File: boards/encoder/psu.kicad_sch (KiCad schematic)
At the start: 10 parts, among them J1 Conn_PWR, U2 TPS62A02A

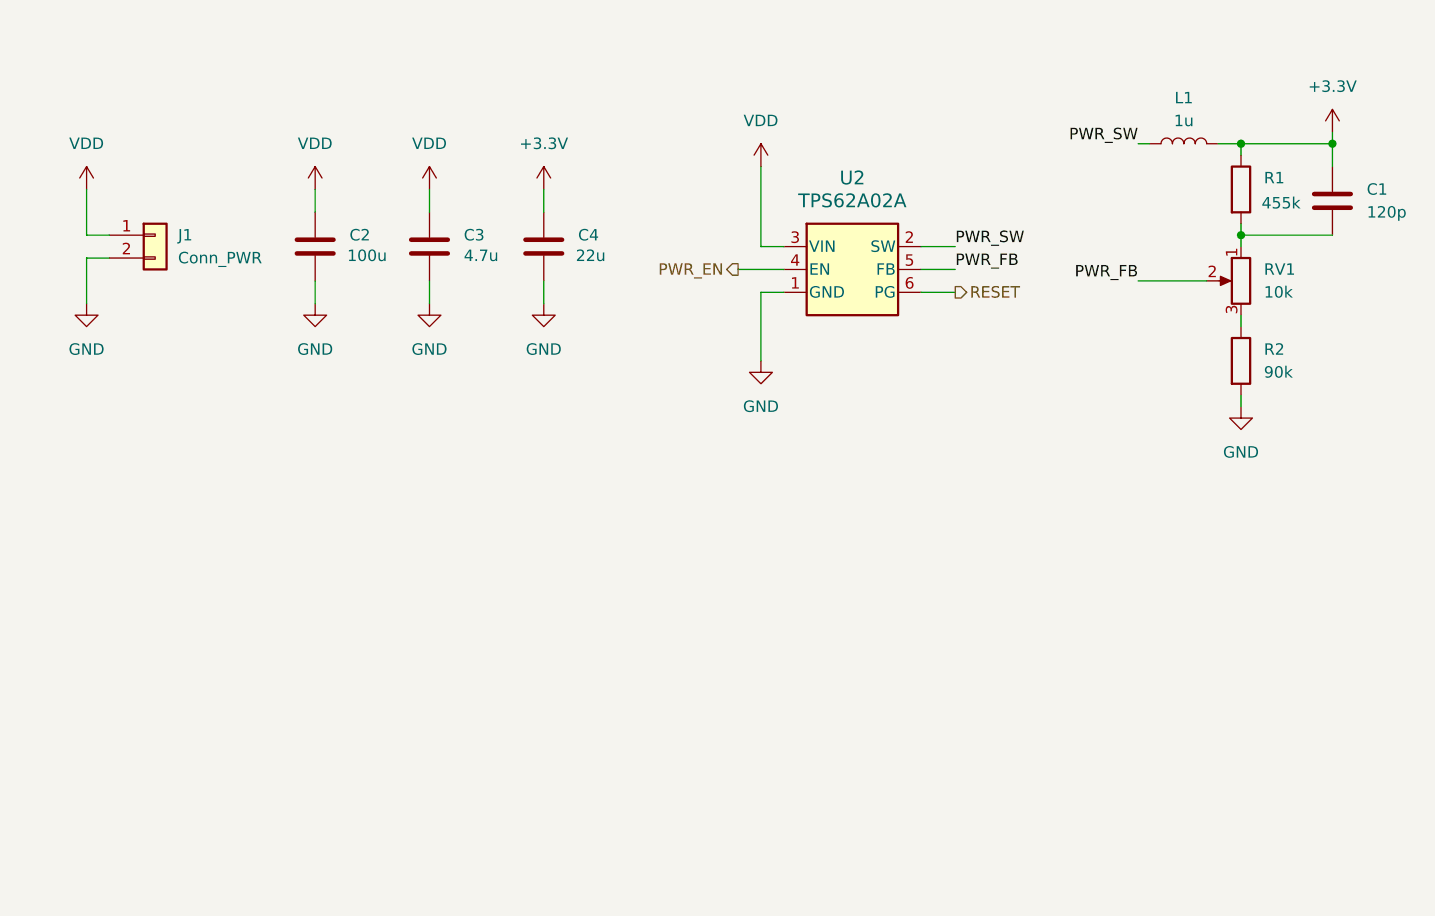
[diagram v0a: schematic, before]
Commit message: v0.1.18
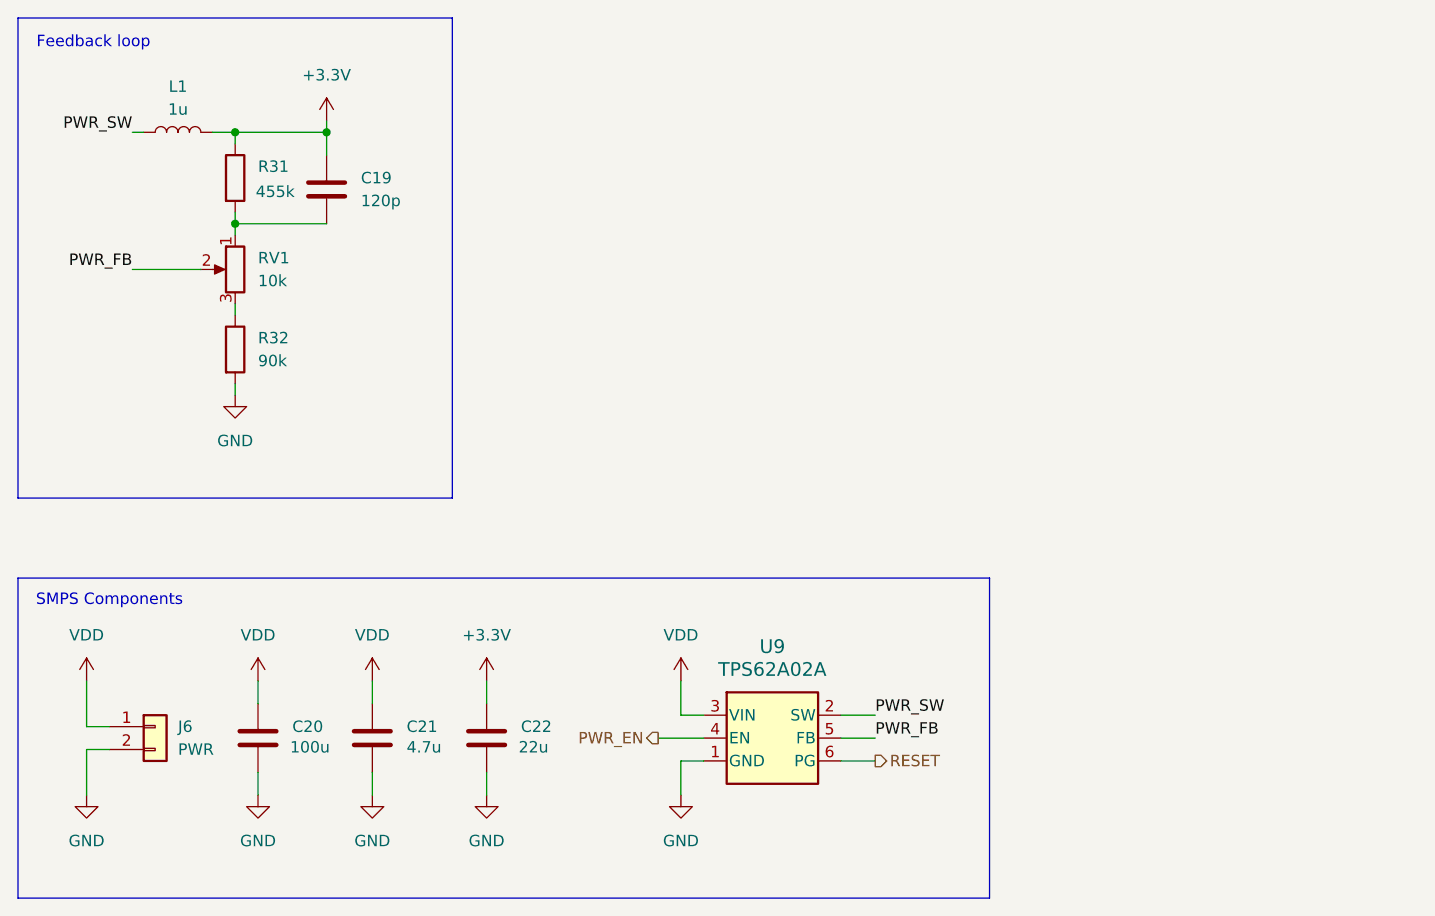
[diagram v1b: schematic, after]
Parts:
- J6: renamed from J1; value Conn_PWR -> PWR
- renumbered C1 to C19, C2 to C20, C3 to C21, C4 to C22, R1 to R31, R2 to R32, U2 to U9
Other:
- note added: "Feedback loop"
- note added: "SMPS Components"
- company: (none) -> MetisVela
- title: (none) -> Wanda
- moved on the sheet: C19, C20, C21, C22, J6, L1, R31, R32, RV1, U9
